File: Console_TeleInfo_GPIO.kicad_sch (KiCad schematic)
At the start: 6 parts, among them J13 Conn_02x06_Odd_Even

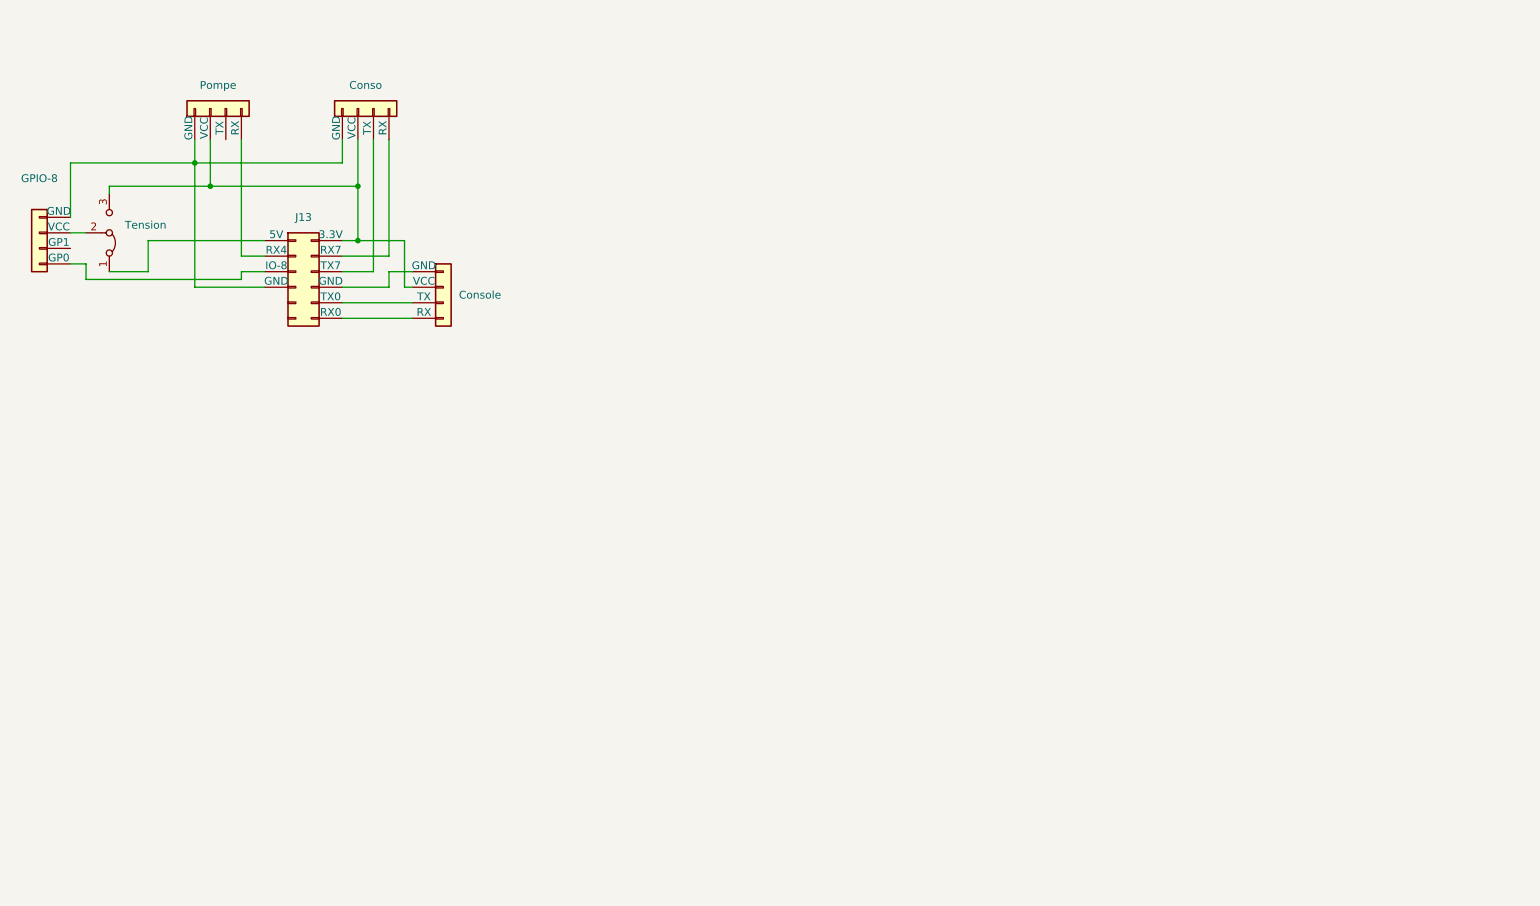
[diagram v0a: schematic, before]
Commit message: Finalize the schema
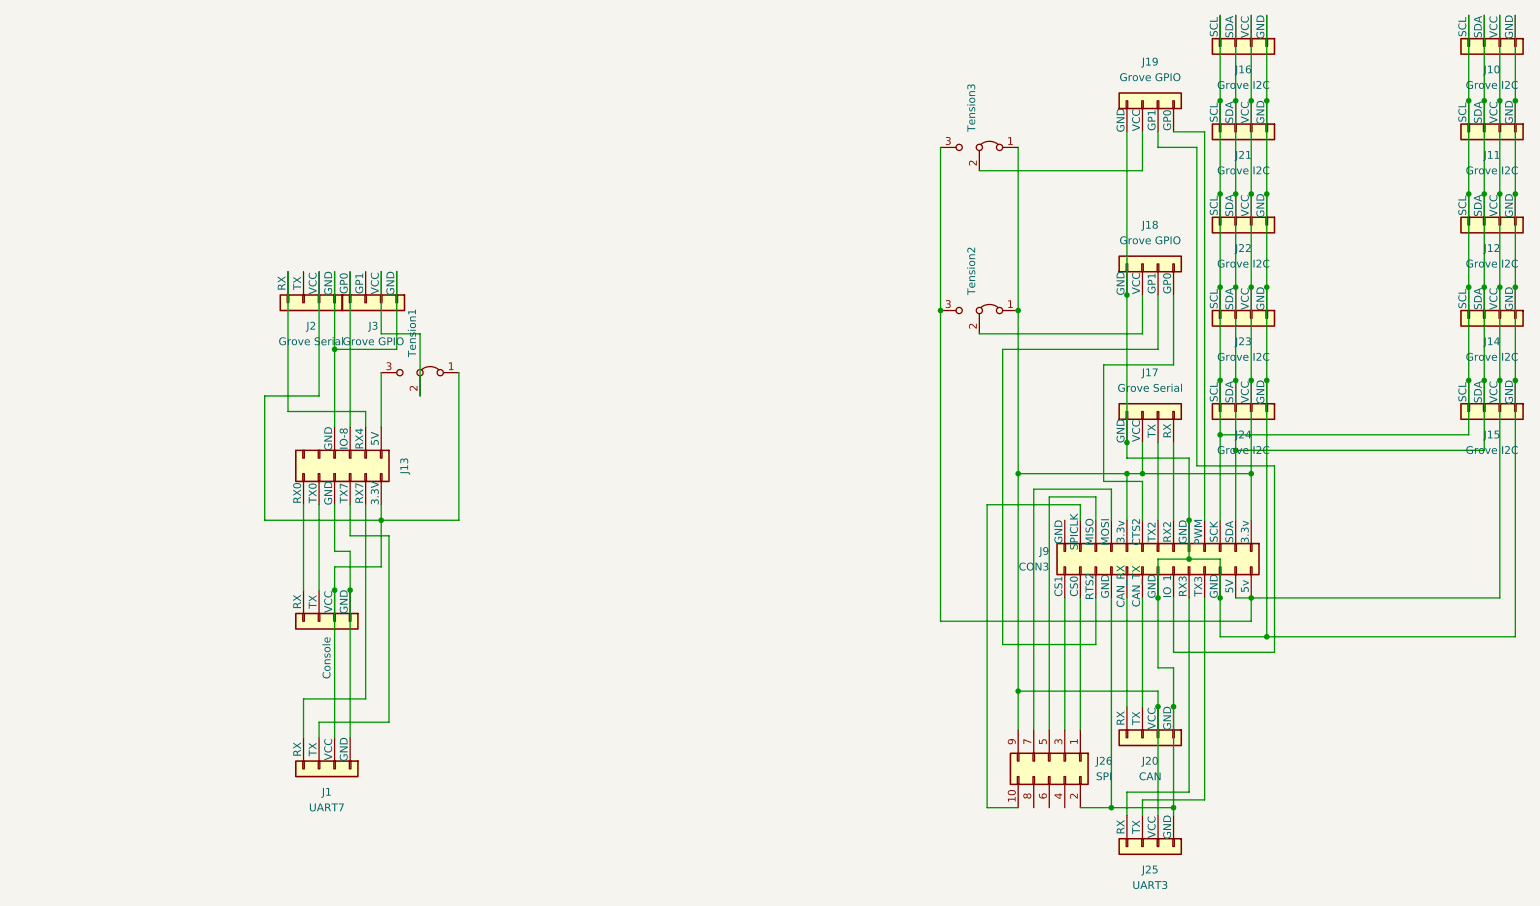
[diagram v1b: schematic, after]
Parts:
- removed Conso, Pompe: Grove Serial, symbol BananaPI:Grove_Serial
- removed GPIO-8: Grove GPIO, symbol BananaPI:Grove_GPIO
- removed Tension: Jumper_3_Bridged12, symbol Jumper:Jumper_3_Bridged12
- added J1: UART7, symbol BananaPI:Grove_Serial
- added J10, J11, J12, J14, J15, J16, J21, J22, J23, J24: Grove I2C, symbol BananaPI:Grove_I2C
- added J17, J2: Grove Serial, symbol BananaPI:Grove_Serial
- added J18, J19, J3: Grove GPIO, symbol BananaPI:Grove_GPIO
- added J20: CAN, symbol BananaPI:Grove_Serial
- added J25: UART3, symbol BananaPI:Grove_Serial
- added J26: SPI, symbol Connector_Generic:Conn_02x05_Odd_Even
- added J9: CON3, symbol BananaPI:CON3
- added Tension1, Tension2, Tension3: Jumper_3_Bridged12, symbol Jumper:Jumper_3_Bridged12
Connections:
- net at Console.1 (GND), J13.8 (GND): now also J1.1 (GND)
- net at Console.2 (VCC), J13.2 (3.3V): now also J1.2 (VCC), J2.2 (VCC), Tension1.1 (A)
- net at J13.1 (5V): now also Tension1.3 (B)
- net at J13.3 (RX4): now also J2.4 (RX)
- net at J13.4 (RX7): now also J1.4 (RX)
- net at J13.5 (IO-8): now also J3.4 (GP0)
- net at J13.6 (TX7): now also J1.3 (TX)
- net at J13.7 (GND): now also J2.1 (GND), J3.1 (GND)
- new net: J10.1 (GND), J11.1 (GND), J12.1 (GND), J14.1 (GND), J15.1 (GND), J16.1 (GND), J17.1 (GND), J18.1 (GND), J19.1 (GND), J20.1 (GND), J21.1 (GND), J22.1 (GND), J23.1 (GND), J24.1 (GND), J25.1 (GND), J26.2 (Pin_2), J9.14 (GND), J9.20 (GND), J9.6 (GND), J9.9 (GND)
- new net: J16.2 (VCC), J17.2 (VCC), J20.2 (VCC), J21.2 (VCC), J22.2 (VCC), J23.2 (VCC), J24.2 (VCC), J25.2 (VCC), J26.9 (Pin_9), J9.1 (3.3v), J9.17 (3.3v), Tension2.1 (A), Tension3.1 (A)
- new net: J20.3 (TX), J9.16 (CAN_TX)
- new net: J20.4 (RX), J9.18 (CAN_RX)
- new net: J26.1 (Pin_1), J9.24 (CS0)
- new net: J26.10 (Pin_10), J9.23 (SPICLK)
- new net: J26.3 (Pin_3), J9.26 (CS1)
- new net: J26.5 (Pin_5), J9.21 (MISO)
- new net: J26.7 (Pin_7), J9.19 (MOSI)
- new net: J10.3 (SDA), J11.3 (SDA), J12.3 (SDA), J14.3 (SDA), J15.3 (SDA), J16.3 (SDA), J21.3 (SDA), J22.3 (SDA), J23.3 (SDA), J24.3 (SDA), J9.3 (SDA)
- new net: J10.4 (SCL), J11.4 (SCL), J12.4 (SCL), J14.4 (SCL), J15.4 (SCL), J16.4 (SCL), J21.4 (SCL), J22.4 (SCL), J23.4 (SCL), J24.4 (SCL), J9.5 (SCK)
- new net: J19.2 (VCC), Tension3.2 (C)
- new net: J19.3 (GP1), J9.12 (IO_1)
- new net: J19.4 (GP0), J9.7 (PWM)
- new net: J10.2 (VCC), J11.2 (VCC), J12.2 (VCC), J14.2 (VCC), J15.2 (VCC), J9.2 (5v), J9.4 (5V), Tension2.3 (B), Tension3.3 (B)
- new net: J18.2 (VCC), Tension2.2 (C)
- new net: J18.3 (GP1), J9.22 (RTS2)
- new net: J18.4 (GP0), J9.15 (CTS2)
- new net: J25.3 (TX), J9.8 (TX3)
- new net: J25.4 (RX), J9.10 (RX3)
- new net: J3.2 (VCC), Tension1.2 (C)
- new net: J17.4 (RX), J9.11 (RX2)
- new net: J17.3 (TX), J9.13 (TX2)
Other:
- moved on the sheet: Console, J13
